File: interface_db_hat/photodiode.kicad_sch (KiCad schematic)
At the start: 10 parts, among them J15 Screw_Terminal_01x02, J16 Screw_Terminal_01x02, U10 LM358, U3 BDJ0GA5WEFJ

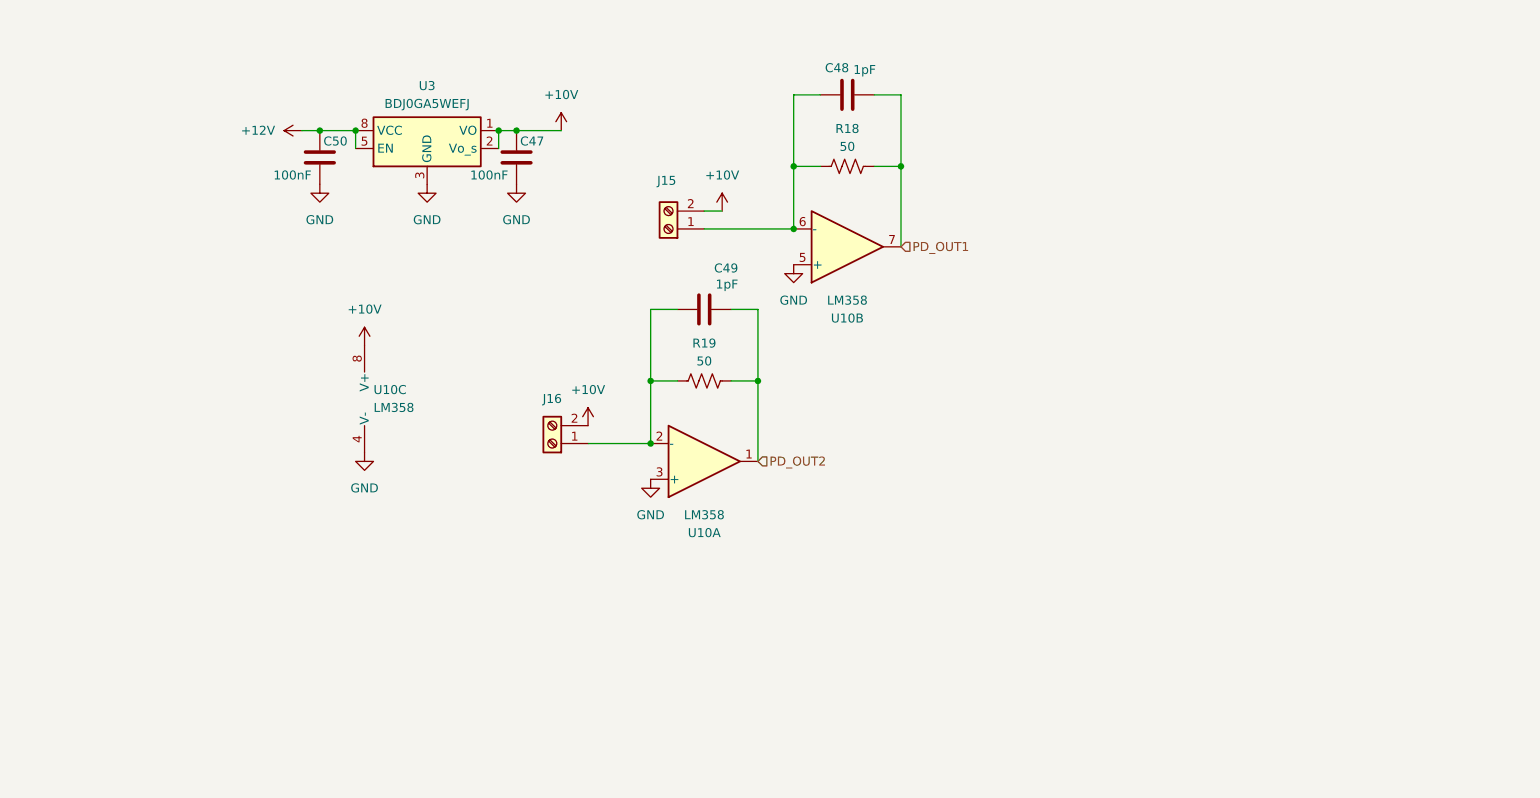
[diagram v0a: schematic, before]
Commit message: update
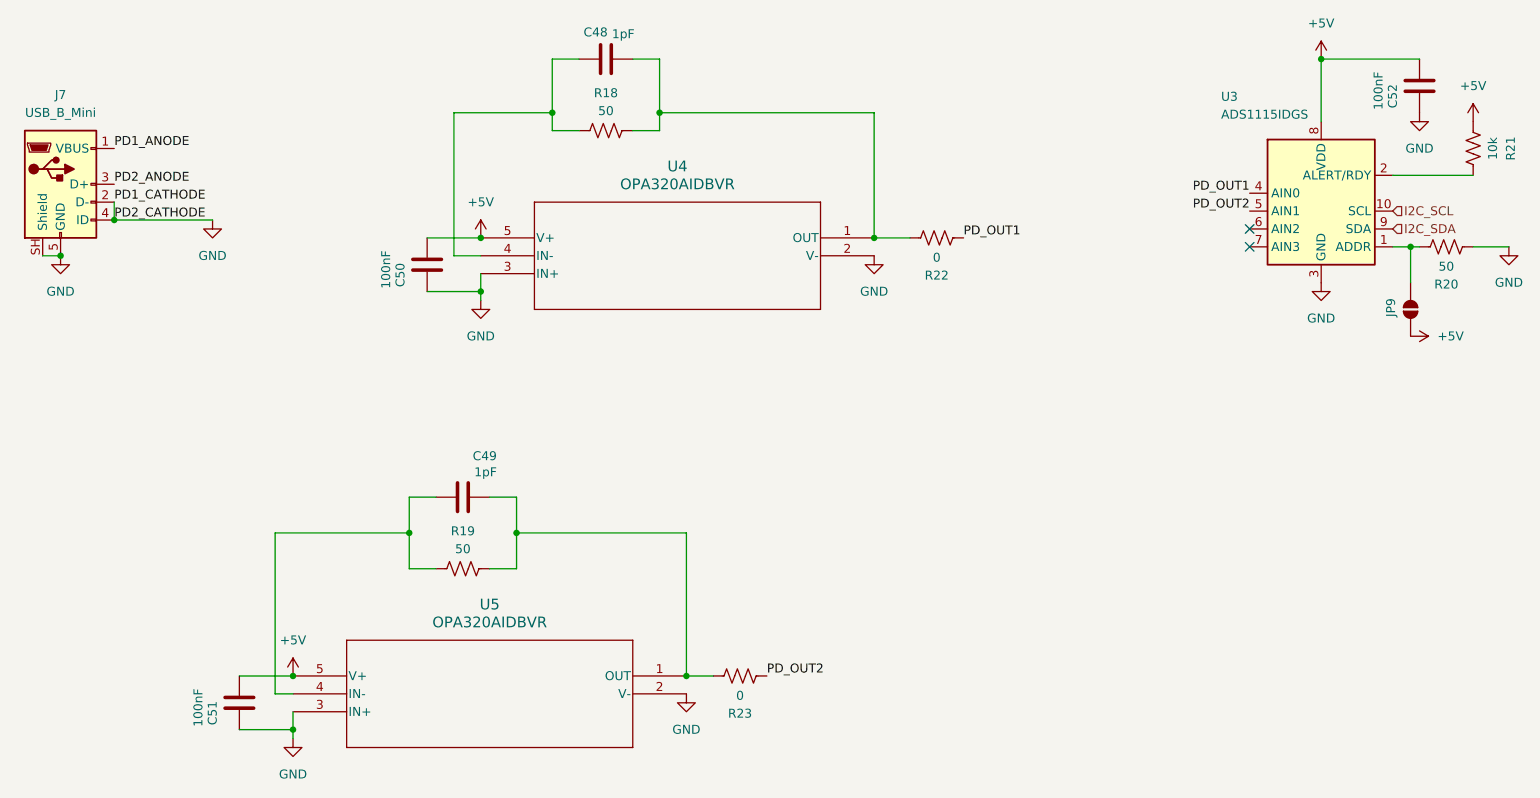
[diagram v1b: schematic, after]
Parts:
- removed C47: 100nF, Capacitor_SMD:C_0603_1608Metric_Pad1.08x0.95mm_HandSolder, symbol Device:C
- removed J15, J16: Screw_Terminal_01x02, Terminal_Block_Custom:1x02_P2.54mm_Horizontal, symbol Connector:Screw_Terminal_01x02
- removed U10: LM358, Package_SO:SOIC-8_3.9x4.9mm_P1.27mm, symbol Amplifier_Operational:LM358
- removed U3: BDJ0GA5WEFJ, Package_SO:HTSOP-8-1EP_3.9x4.9mm_P1.27mm_EP2.4x3.2mm, symbol Regulator_Linear:BDJ0GA5WEFJ
- added C51, C52: 100nF, Capacitor_SMD:C_0603_1608Metric_Pad1.08x0.95mm_HandSolder, symbol Device:C
- added J7: USB_B_Mini, symbol Connector:USB_B_Mini
- added JP9: SolderJumper_2_Open, Jumper:SolderJumper-2_P1.3mm_Open_TrianglePad1.0x1.5mm, symbol Jumper:SolderJumper_2_Open
- added R20: 50, Resistor_SMD:R_0603_1608Metric_Pad0.98x0.95mm_HandSolder, symbol Device:R_US
- added R21: 10k, Resistor_SMD:R_0603_1608Metric_Pad0.98x0.95mm_HandSolder, symbol Device:R_US
- added R22, R23: 0, Resistor_SMD:R_0603_1608Metric_Pad0.98x0.95mm_HandSolder, symbol Device:R_US
- added U3: ADS1115IDGS, Package_SO:TSSOP-10_3x3mm_P0.5mm, symbol Analog_ADC:ADS1115IDGS
- added U4, U5: OPA320AIDBVR, DBV5, symbol OPA320:OPA320AIDBVR
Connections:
- net +12V is gone; now on net GND: C50.2
- net GND: now also C51.2, C52.2, J7.2 (D-), J7.4 (ID), J7.5 (GND), J7.SH (Shield), R20.1, U3.3 (GND), U4.2 (V-), U4.3 (IN+), U5.2 (V-), U5.3 (IN+); no longer C50.1
- net PD_OUT1: now also R22.1, U3.4 (AIN0); no longer C48.1, R18.2
- net PD_OUT2: now also R23.1, U3.5 (AIN1); no longer C49.1, R19.2
- net at C49.2, R19.1: now also U5.4 (IN-)
- net at C48.2, R18.1: now also U4.4 (IN-)
- new net: C48.1, R18.2, R22.2, U4.1 (OUT)
- new net: C49.1, R19.2, R23.2, U5.1 (OUT)
- new net: JP9.1 (A), R20.2, U3.1 (ADDR)
- new net: R21.2, U3.2 (ALERT/RDY)
- new net +5V: C50.1, C51.1, C52.1, JP9.2 (B), R21.1, U3.8 (VDD), U4.5 (V+), U5.5 (V+)
- new net I2C_SCL: U3.10 (SCL)
- new net I2C_SDA: U3.9 (SDA)
- new net PD1_ANODE: J7.1 (VBUS)
- new net PD2_ANODE: J7.3 (D+)
- no-connect marks 0 -> 2
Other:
- moved on the sheet: C48, C49, R18, R19
